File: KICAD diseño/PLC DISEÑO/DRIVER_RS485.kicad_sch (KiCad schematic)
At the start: 1 part

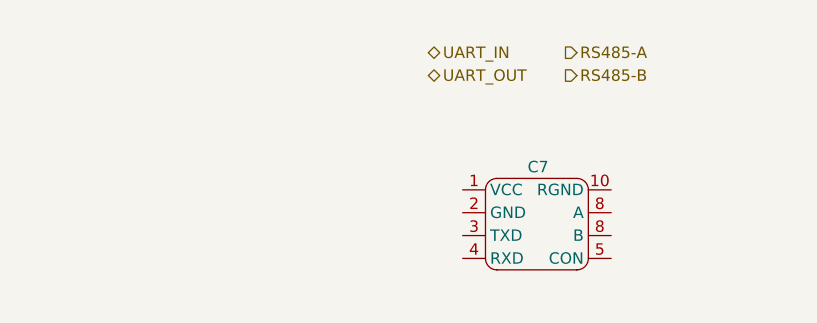
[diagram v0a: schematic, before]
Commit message: Actualizacion
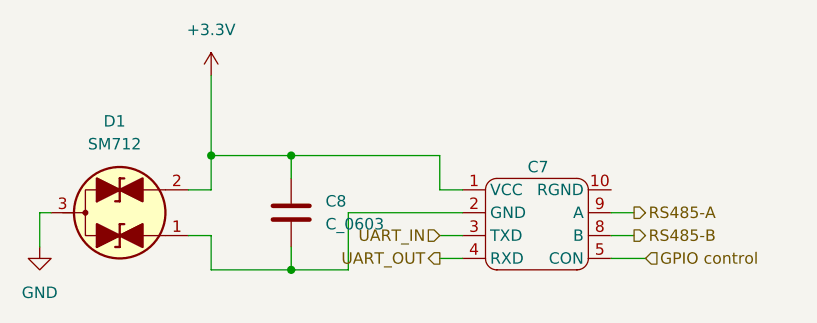
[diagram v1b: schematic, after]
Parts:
- added C8: C_0603, PCM_Capacitor_SMD_AKL:C_0603_1608Metric, symbol PCM_Capacitor_AKL:C_0603
- added D1: SM712, PCM_Package_TO_SOT_SMD_AKL:SOT-23, symbol PCM_Diode_TVS_AKL:SM712
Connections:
- net RS485-A: now also C7.9 (A)
- net RS485-B: now also C7.8 (B)
- net UART_IN: now also C7.3 (TXD)
- net UART_OUT: now also C7.4 (RXD)
- net +3.3V: now reaches C7.1 (VCC)
- net +3.3V: now also C8.1, D1.2 (A2)
- net at C7.2 (GND): now also C8.2, D1.1 (A1)
- net GPIO control: now reaches C7.5 (CON)
- new net GND: D1.3 (Com)
